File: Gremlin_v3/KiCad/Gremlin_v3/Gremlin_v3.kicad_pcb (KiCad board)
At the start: 2 copper layers, 92 x 112.8 mm, 55 parts, among them J1 JST_02, J2 5034800540, SW1 Switch, SW2 SW_SPST, U1 Nice_Nano_V2

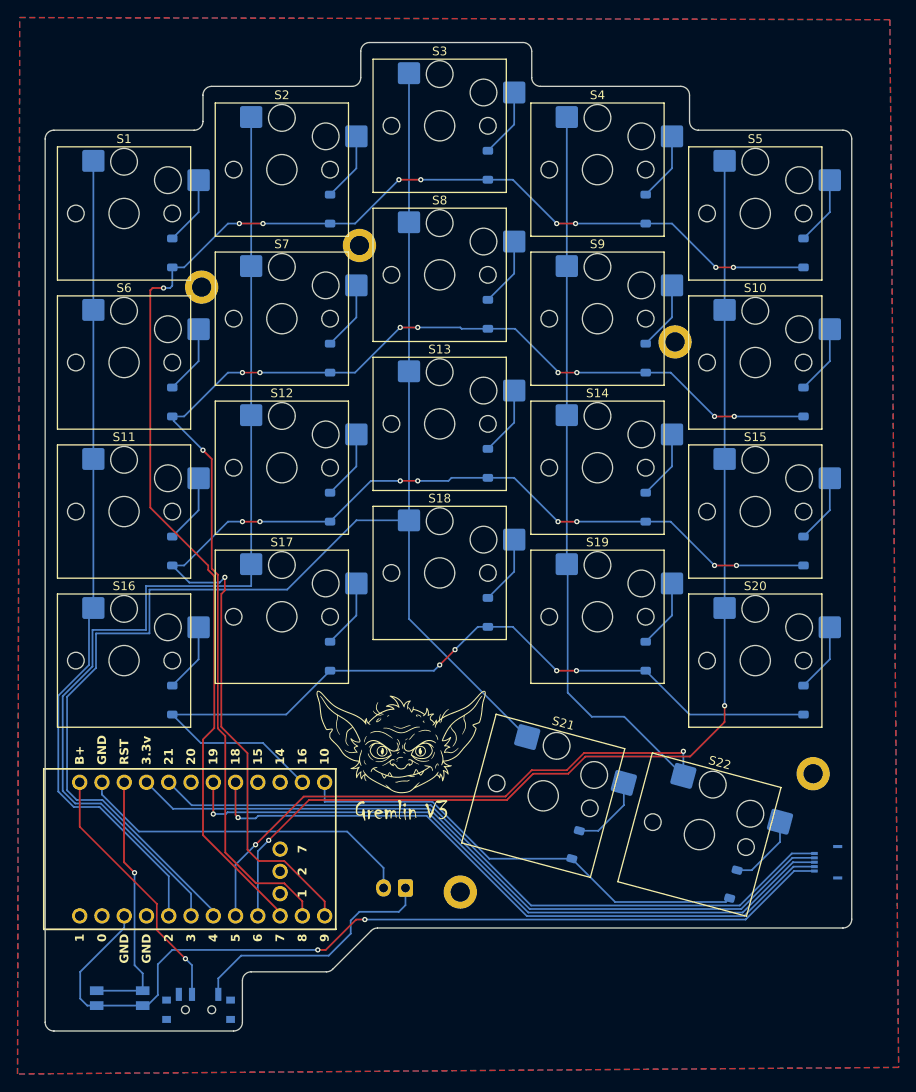
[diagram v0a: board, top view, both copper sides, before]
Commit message: Updated PCB design for CNC Milling
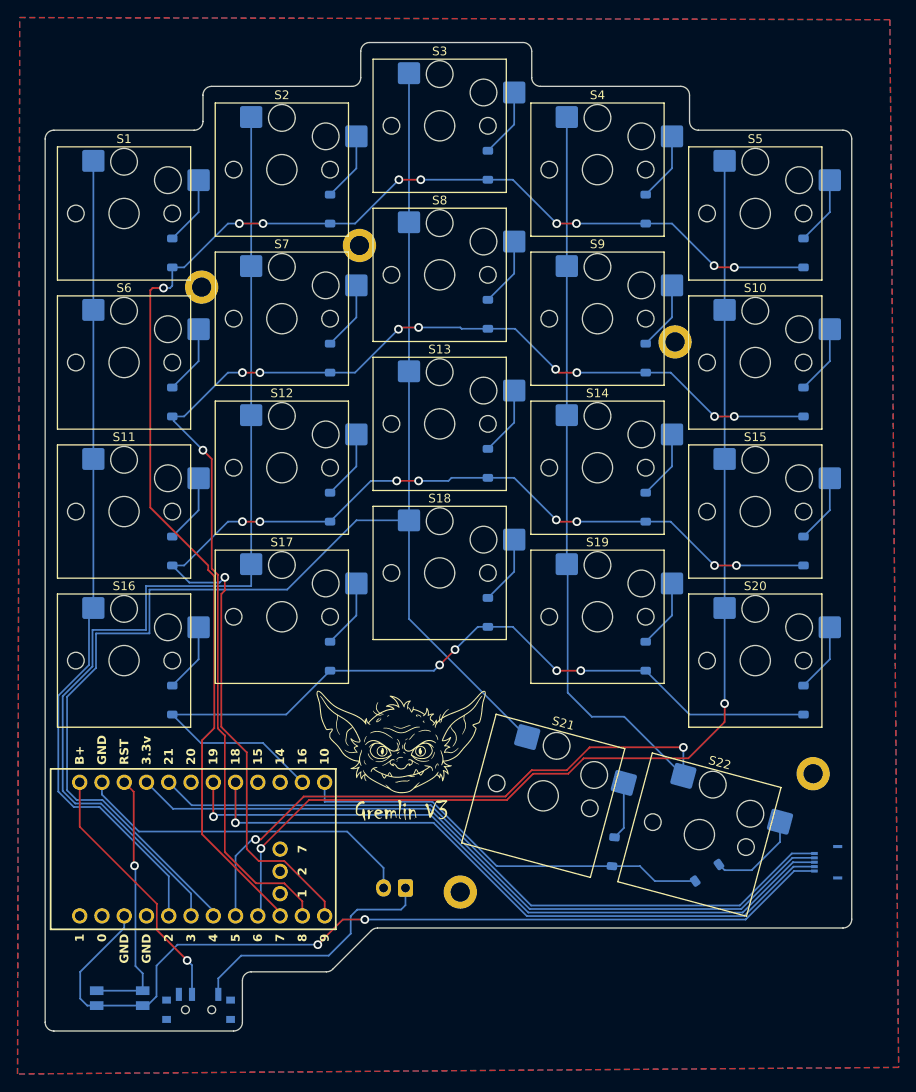
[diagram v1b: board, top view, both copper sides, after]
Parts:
- moved D21 4.37 mm to (164.2, 131.4), turned to 85 degrees
- moved D22 3.27 mm to (174.9, 133.8), turned to 35 degrees
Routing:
- net Row 4: track 53.3 -> 48.2 mm
- net Net-(D22-A): track 8.53 -> 10.9 mm
- net Net-(D21-A): track 8.83 -> 6.64 mm
- net Col 3: track 147.9 -> 149.1 mm
